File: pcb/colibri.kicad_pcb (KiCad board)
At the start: 2 copper layers, 175.2 x 95.1 mm, 91 parts

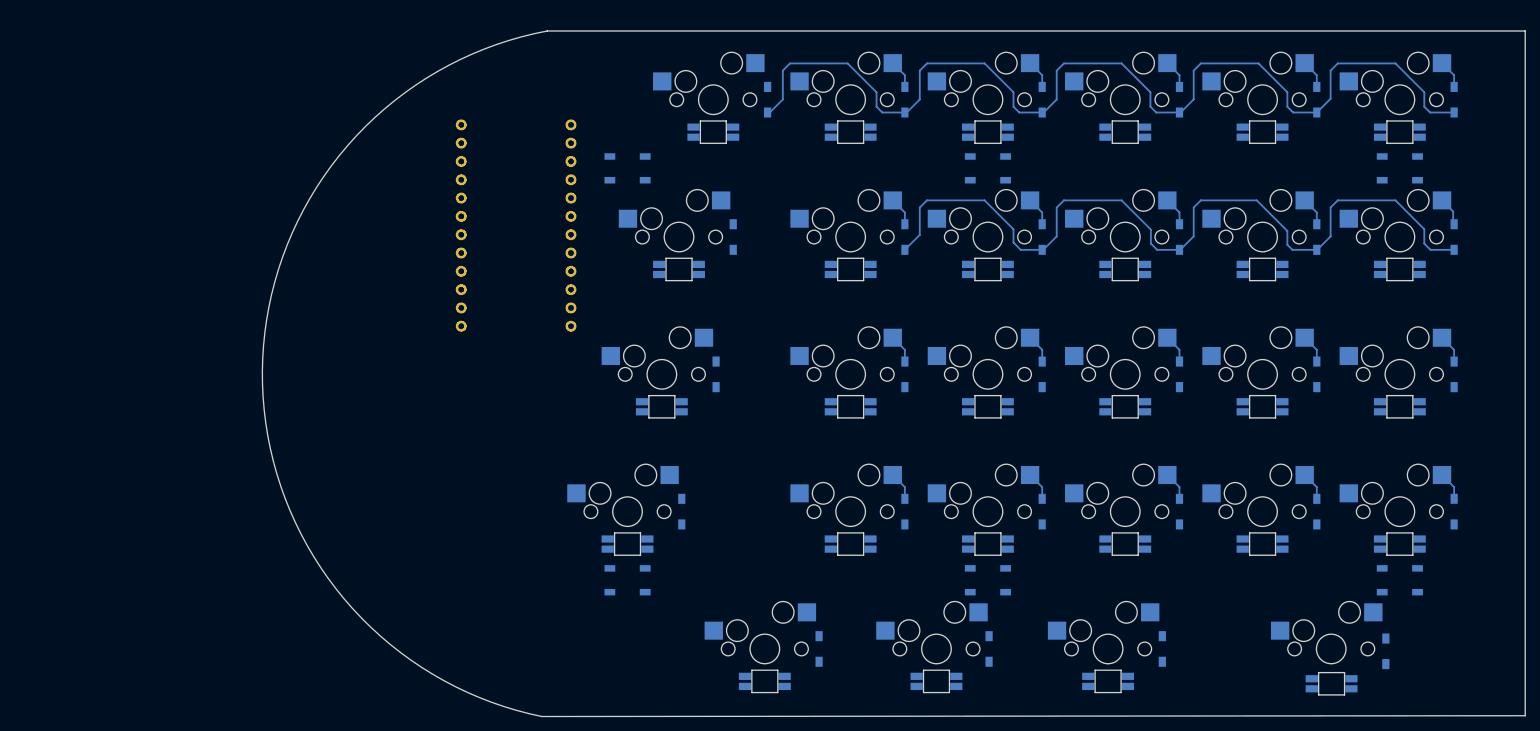
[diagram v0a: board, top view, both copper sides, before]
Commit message: board size
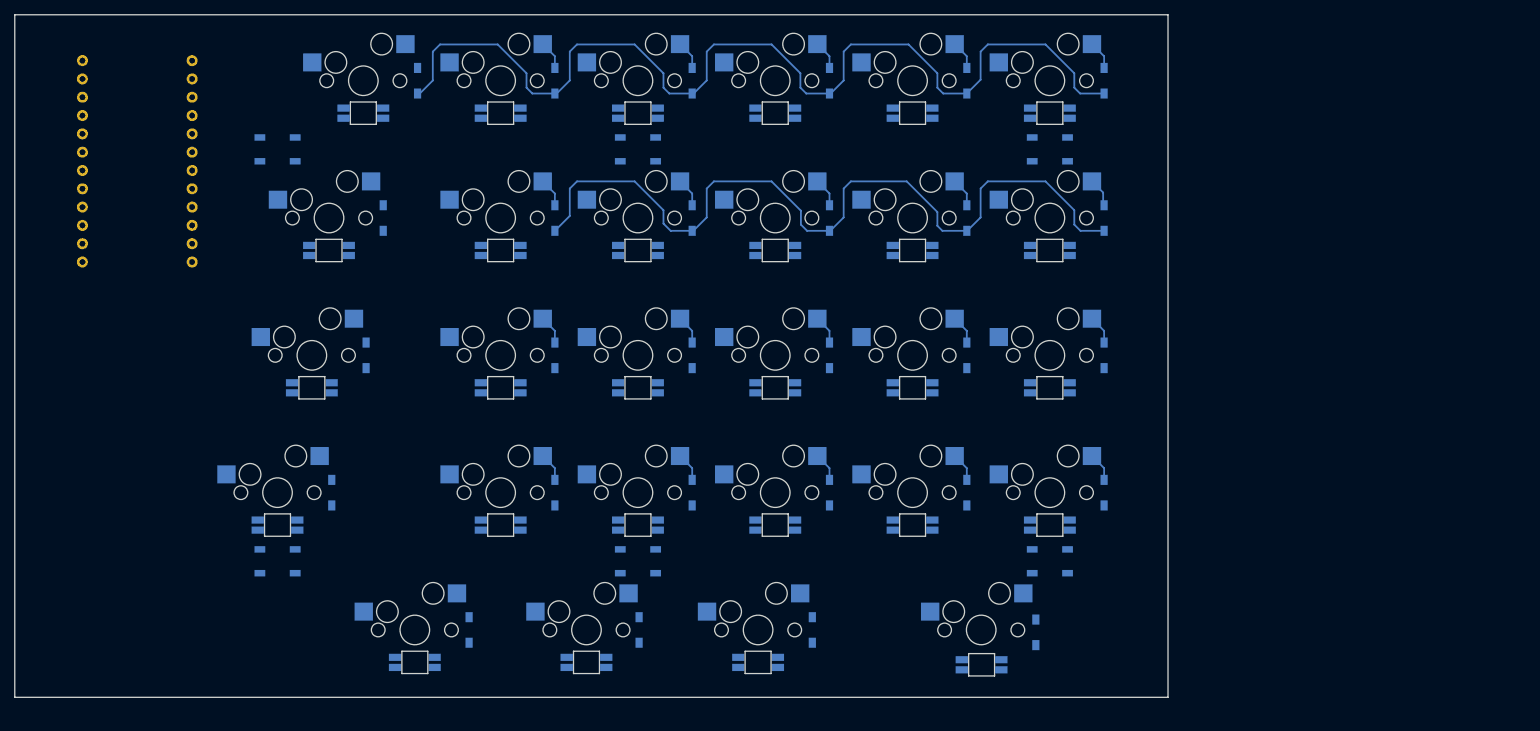
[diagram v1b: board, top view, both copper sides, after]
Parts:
- moved pro-micro1 53.3 mm to (37.4, 61.1)
- moved ld-10 48.6 mm to (133.5, 68.5)
- moved ld-12 48.6 mm to (171.6, 68.5)
- moved ld-14 48.6 mm to (95.4, 87.5)
- moved ld-16 48.6 mm to (133.5, 87.5)
- moved ld-18 48.6 mm to (171.6, 87.5)
- moved ld-19 48.6 mm to (64.4, 106.5)
- moved ld-2 48.6 mm to (95.4, 49.4)
- moved ld-20 48.6 mm to (95.4, 106.5)
- moved ld-22 48.6 mm to (133.5, 106.5)
- moved ld-24 48.6 mm to (171.6, 106.5)
- moved ld-25 48.6 mm to (83.5, 125.6)
- moved ld-27 48.6 mm to (131.1, 125.6)
- moved ld-4 48.6 mm to (133.5, 49.4)
- moved ld-6 48.6 mm to (171.6, 49.4)
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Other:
- board size 175.2 x 95.1 mm -> 160 x 94.7 mm
